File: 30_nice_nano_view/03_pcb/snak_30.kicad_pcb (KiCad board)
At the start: 2 copper layers, 114 x 100.2 mm, 164 parts

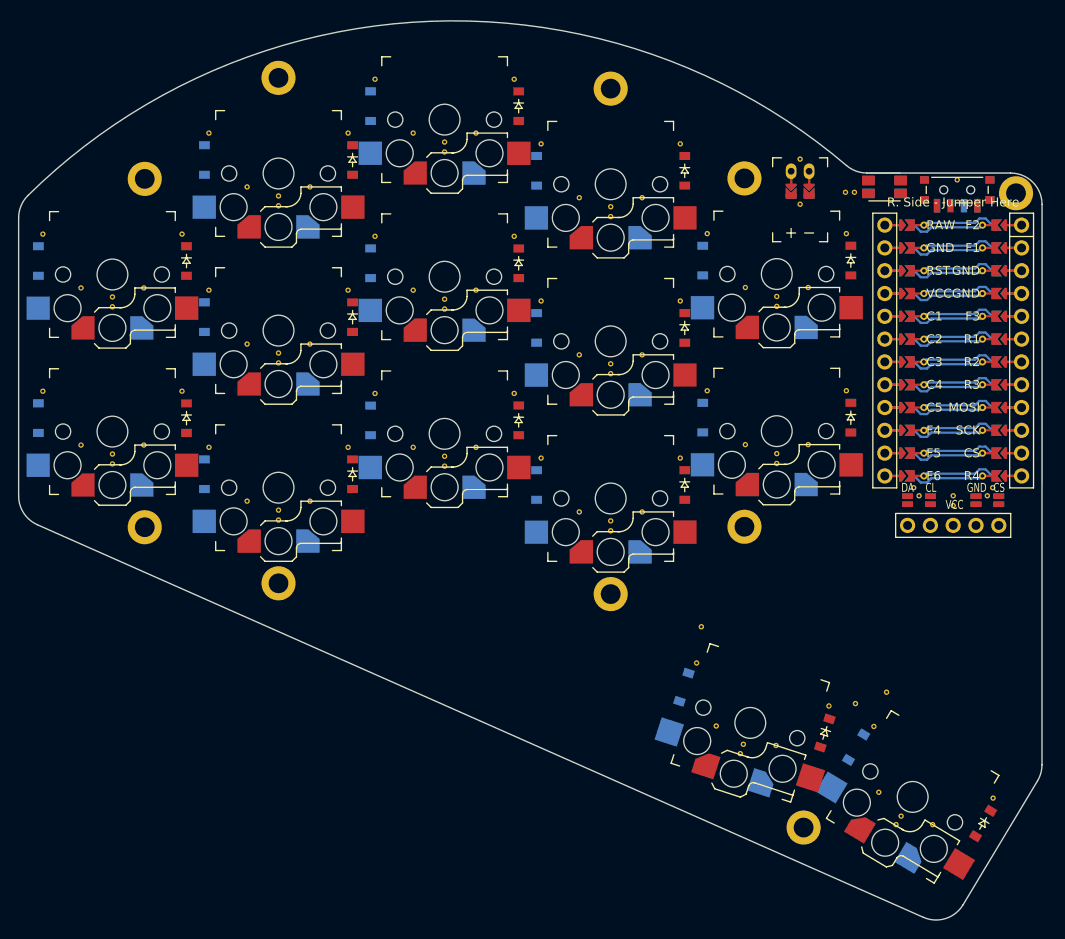
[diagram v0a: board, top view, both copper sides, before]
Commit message: update
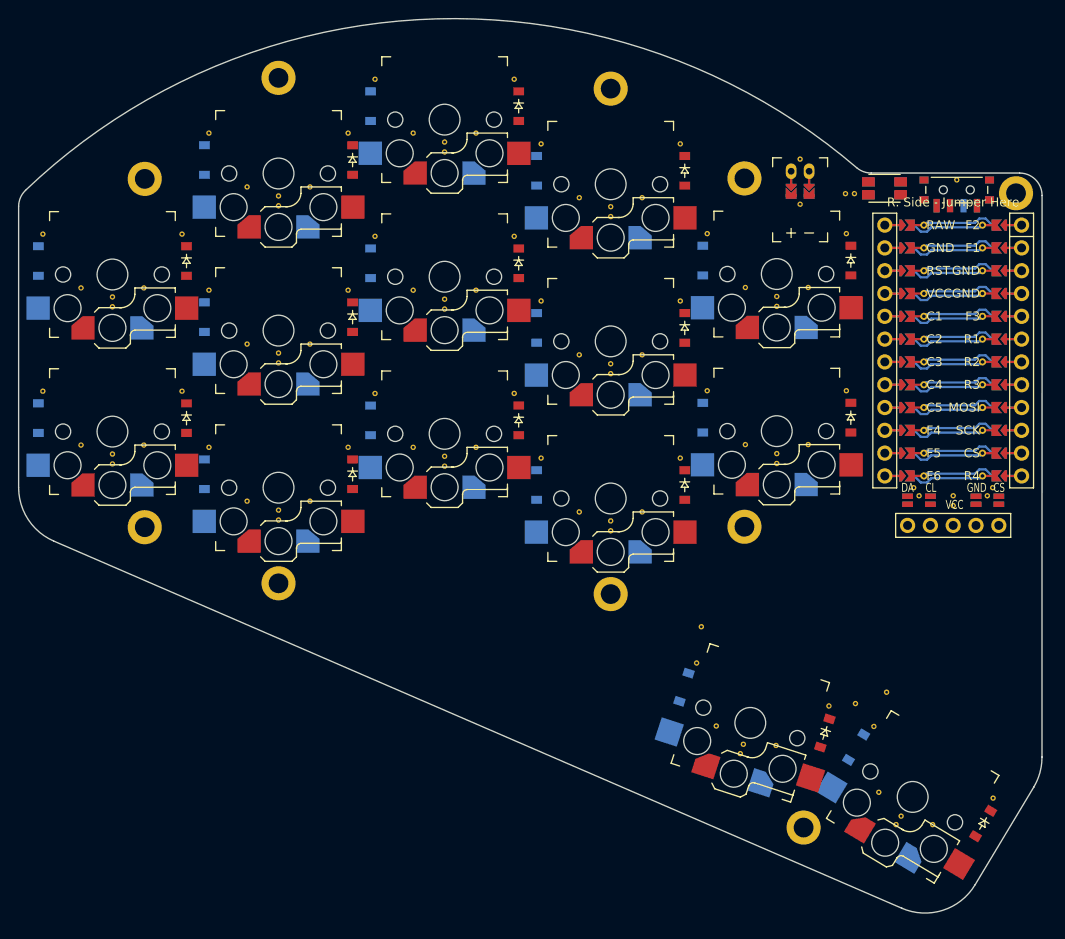
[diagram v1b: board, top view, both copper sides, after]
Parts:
- removed the REF** at (194.1, 54.5)
- removed the REF** at (181.7, 55.8)
- removed the REF** at (182.7, 55.8)
- added REF**: VIA-0.6mm, VIA-0.6mm, F.Cu at (194.1, 54.5)
- added REF**: VIA-0.6mm, VIA-0.6mm, F.Cu at (181.7, 56.0)
- added REF**: VIA-0.6mm, VIA-0.6mm, F.Cu at (182.7, 56.0)
- moved SW2 0.15 mm to (186.0, 55.4)
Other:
- board size 114 x 100.2 mm -> 114 x 99.6 mm
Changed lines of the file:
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@@
   (page A3)
   (title_block
-    (title snak)
+    (title snak_30)
     (rev 0.2.1)
     (company JackMatanky)
@@
       )
       (module power_switch (layer F.Cu)
-        (at 194.1 55.6 90)
+        (at 194.05 55.6 90)
         (attr smd)
         (fp_text reference "SW1" (at -3.6 0 0) (layer F.SilkS) hide
@@
       )
       (module VIA-0.6mm (layer F.Cu)
-      (at 194.1 54.4625 90)
+      (at 194.05 54.4625 90)
       (fp_text reference REF** (at 0 1.4) (layer F.SilkS) hide (effects (font (size 1 1) (thickness 0.15))))
       (fp_text value VIA-0.6mm (at 0 -1.4) (layer F.Fab) hide (effects (font (size 1 1) (thickness 0.15))))
@@
       )
         (module sw_reset_side (layer F.Cu)
-          (at 186 55.25 90)
+          (at 186 55.400000000000006 90)
           (attr smd)
           (fp_text reference "SW2" (at 0 3.5 90) (layer F.SilkS) hide
@@
         )
       (module VIA-0.6mm (layer F.Cu)
-      (at 181.65 55.845 90)
+      (at 181.65 55.995000000000005 90)
       (fp_text reference REF** (at 0 1.4) (layer F.SilkS) hide (effects (font (size 1 1) (thickness 0.15))))
       (fp_text value VIA-0.6mm (at 0 -1.4) (layer F.Fab) hide (effects (font (size 1 1) (thickness 0.15))))
@@
       )
       (module VIA-0.6mm (layer F.Cu)
-      (at 182.65 55.845 90)
+      (at 182.65 55.995000000000005 90)
       (fp_text reference REF** (at 0 1.4) (layer F.SilkS) hide (effects (font (size 1 1) (thickness 0.15))))
       (fp_text value VIA-0.6mm (at 0 -1.4) (layer F.Fab) hide (effects (font (size 1 1) (thickness 0.15))))
@@
                 (fp_circle (center 0 0) (end -2.1500000000000004 0) (layer B.CrtYd) (width 0.05))
             )
-            (gr_line (start 190.3330289052461 136.60645643375523) (end 91.63212207196788 92.87257788445723) (angle 90) (layer Edge.Cuts) (width 0.15))
-(gr_line (start 89.55 89.67263689687813) (end 89.55 58.6923717) (angle 90) (layer Edge.Cuts) (width 0.15))
-(gr_line (start 184.0390866 53.7) (end 200.04959101968365 53.7) (angle 90) (layer Edge.Cuts) (width 0.15))
-(gr_line (start 203.54959101969533 57.20040880027227) (end 203.542299481328 119.60772958095185) (angle 90) (layer Edge.Cuts) (width 0.15))
-(gr_line (start 203.04238504591765 121.40995413963924) (end 194.75099239794127 135.20914880498668) (angle 90) (layer Edge.Cuts) (width 0.15))
-(gr_arc (start 93.05 89.67263689687813) (end 89.55 89.67263689687813) (angle -66.10210628397607) (layer Edge.Cuts) (width 0.15))
-(gr_arc (start 200.04959101968365 57.2) (end 203.54959101968365 57.200408800000005) (angle -90.00669215147377) (layer Edge.Cuts) (width 0.15))
-(gr_arc (start 200.04229948131632 119.60732078086585) (end 203.04238498131633 121.40995408086584) (angle -30.993309104513855) (layer Edge.Cuts) (width 0.15))
-(gr_arc (start 191.7509068332782 133.40651544617617) (end 190.3330289332782 136.60645644617617) (angle -82.89789246308536) (layer Edge.Cuts) (width 0.15))
-(gr_arc (start 138 104.25) (end 181.76955420000002 52.8644366) (angle -85.0392721574179) (layer Edge.Cuts) (width 0.15))
-(gr_arc (start 93.05 58.6923717) (end 90.59179689999999 56.200938900000004) (angle -45.38465281566448) (layer Edge.Cuts) (width 0.15))
-(gr_arc (start 184.0390866 50.2) (end 181.7695542 52.864436600000005) (angle -40.423924973082364) (layer Edge.Cuts) (width 0.15))
+            (gr_line (start 187.9361383126695 135.5973361797826) (end 93.46742259266699 94.6960902216509) (angle 90) (layer Edge.Cuts) (width 0.15))
+(gr_line (start 89.55 88.73116825471402) (end 89.55 57.4287248) (angle 90) (layer Edge.Cuts) (width 0.15))
+(gr_line (start 184.5162338 53.7) (end 201.04970787119927 53.7) (angle 90) (layer Edge.Cuts) (width 0.15))
+(gr_line (start 203.54970787121096 56.20029199984856) (end 203.54239666528505 118.77594483550638) (angle 90) (layer Edge.Cuts) (width 0.15))
+(gr_line (start 202.61398412985187 122.12293299453017) (end 196.0903029356296 132.980161756421) (angle 90) (layer Edge.Cuts) (width 0.15))
+(gr_arc (start 96.05 88.73116825471402) (end 89.55 88.73116825471402) (angle -66.58927965288365) (layer Edge.Cuts) (width 0.15))
+(gr_arc (start 197.04239666528505 118.77518543577753) (end 202.61398416528505 122.12293293577753) (angle -30.993305013330712) (layer Edge.Cuts) (width 0.15))
+(gr_arc (start 190.51871551511385 129.63241412413697) (end 187.93613841511385 135.59733622413697) (angle -82.4107158960997) (layer Edge.Cuts) (width 0.15))
+(gr_arc (start 138 105.5) (end 182.889792 53.0986014) (angle -84.29262829616823) (layer Edge.Cuts) (width 0.15))
+(gr_arc (start 92.05 57.4287248) (end 90.3225564 55.621534) (angle -46.29246811148599) (layer Edge.Cuts) (width 0.15))
+(gr_arc (start 184.5162338 51.2) (end 182.88979210000002 53.0986014) (angle -40.58509640765422) (layer Edge.Cuts) (width 0.15))
+(gr_arc (start 201.04970787119927 56.2) (end 203.54970787119927 56.200292000000005) (angle -90.00669214354576) (layer Edge.Cuts) (width 0.15))
+(gr_arc (start 201.04239666528505 118.77565283577754) (end 203.54239666528505 118.77594493577753) (angle -0.000002871003403015493) (layer Edge.Cuts) (width 0.15))
+(gr_arc (start 200.47106586528506 120.83533773577753) (end 202.61398406528505 122.12293293577753) (angle -0.0000012278021017664287) (layer Edge.Cuts) (width 0.15))
+(gr_arc (start 188.92943731511386 133.30313542413697) (end 187.93613831511385 135.59733622413697) (angle -0.0000031980794119590428) (layer Edge.Cuts) (width 0.15))
 (gr_circle (center 103.6 54.35) (end 104.6 54.35) (layer Eco1.User) (width 0.15))
 (gr_circle (center 103.6 93.15) (end 104.6 93.15) (layer Eco1.User) (width 0.15))
